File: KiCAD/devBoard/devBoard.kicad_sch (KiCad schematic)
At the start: 10 parts, among them J1 ATmega88{slash}328{slash}328P, J2 ATtiny4313, J3 ATtiny85, J4 ZIF Socket, Y1 Crystal

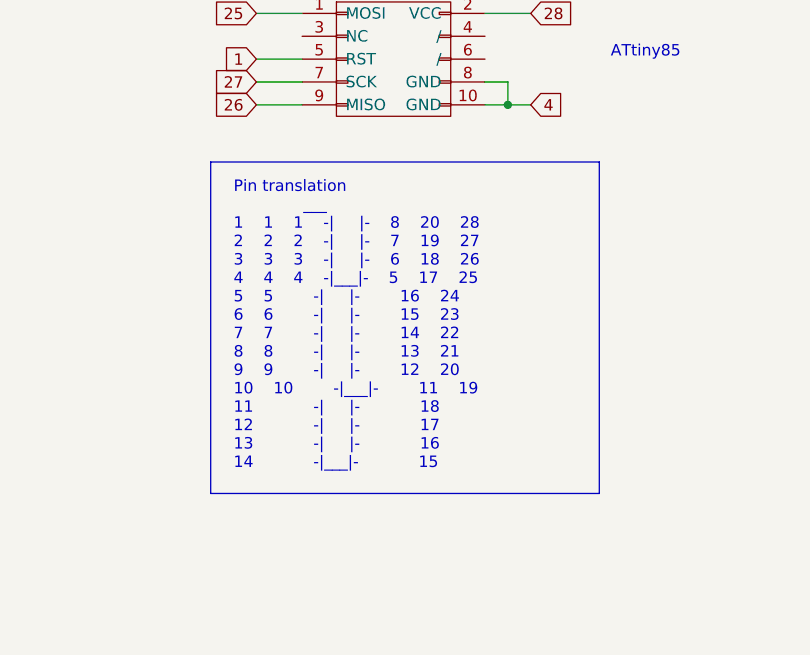
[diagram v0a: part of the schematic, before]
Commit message: new kicad version
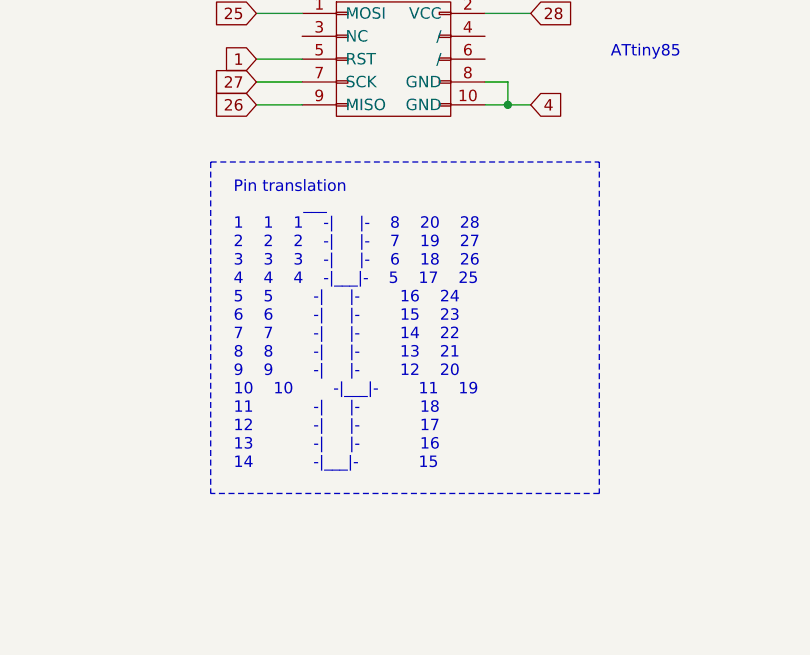
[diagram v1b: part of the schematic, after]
